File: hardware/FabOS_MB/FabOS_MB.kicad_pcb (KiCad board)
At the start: 4 copper layers, 68 x 68 mm, 117 parts, among them J201 USB_A, J301 RJ45, J401 USB_C_Receptacle, J601 Conn_ST_STDC14, SW601 boot, SW602 SW_Push, SW603 SW_Push, SW604 SW_Push, SW605 SW_Push, U201 NCV7329, U301 LAN8742A, U302 CND-tek B1601S, U303 USBLC6-4SC6, U401 USBLC6-2SC6, U501 TDPOWER TAS12-5-W2, U502 TPS563201, U601 STM32F407VETx, Y301 Crystal_GND24

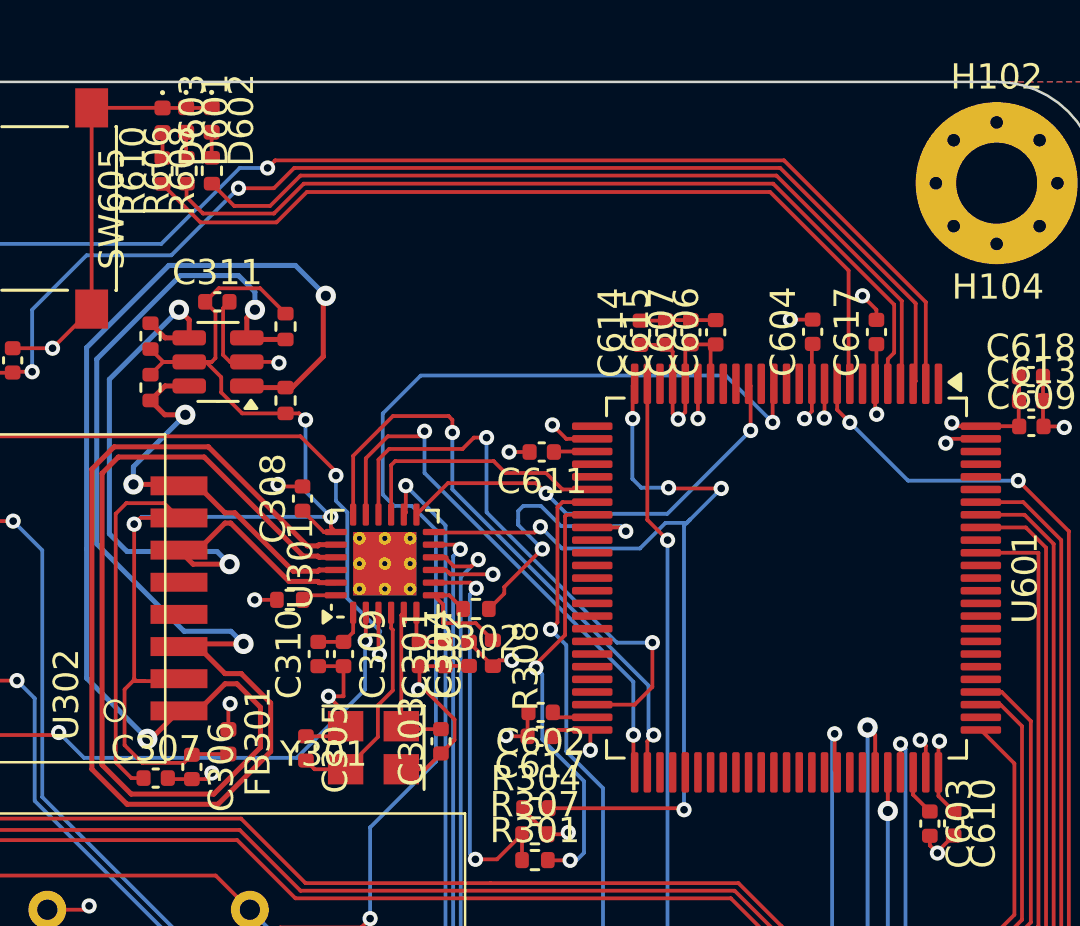
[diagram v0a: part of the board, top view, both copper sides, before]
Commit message: update
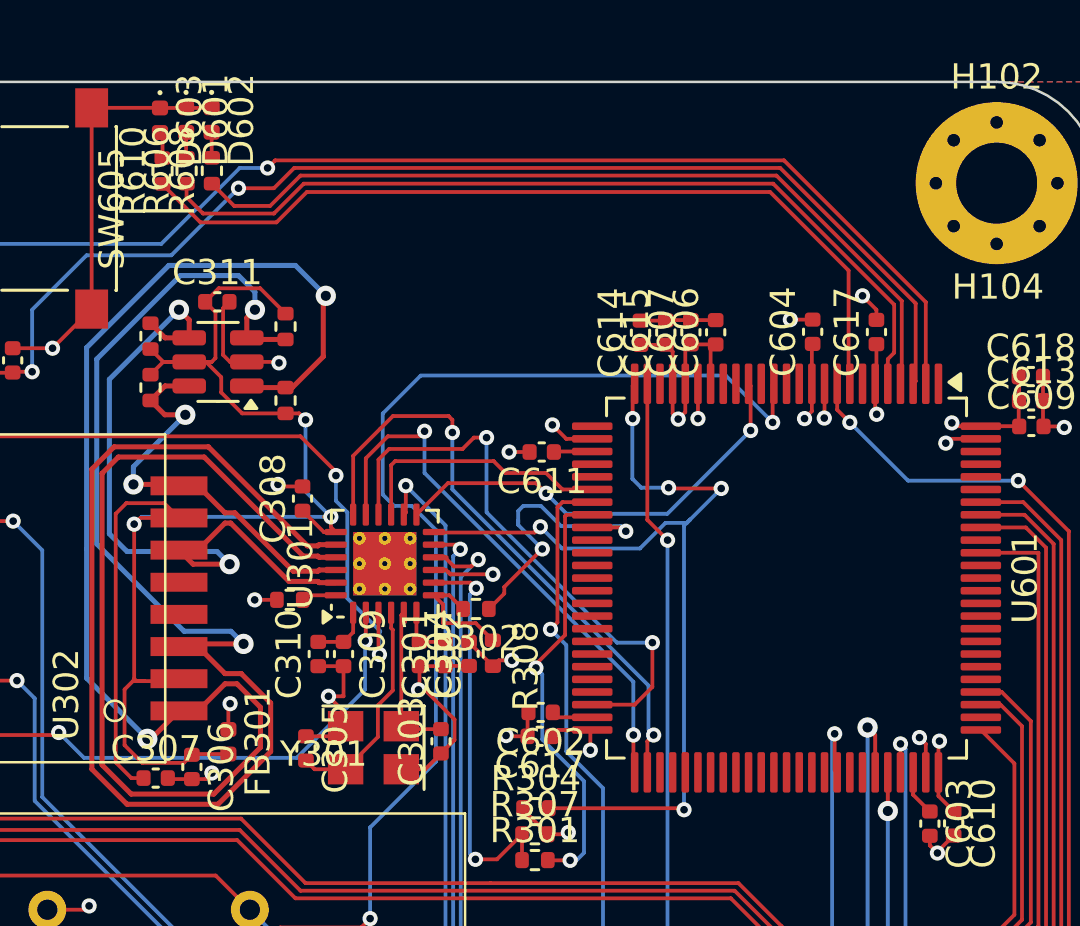
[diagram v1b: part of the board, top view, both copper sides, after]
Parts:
- moved D603 0.10 mm to (127.0, 97.5)
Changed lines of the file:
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@@
 	(footprint "Diode_SMD:D_0402_1005Metric"
 		(layer "F.Cu")
-		(at 127.05 97.515 -90)
+		(at 126.95 97.515 -90)
 		(descr "Diode SMD 0402 (1005 Metric), square (rectangular) end terminal, IPC_7351 nominal, (Body size source: http://www.tortai-tech.com/upload/download/2011102023233369053.pdf), generated with kicad-footprint-generator")
 		(tags "diode")
@@
 	)
 	(segment
+		(start 156.95 121.9)
+		(end 157.2 122.15)
+		(width 0.15)
+		(layer "F.Cu")
+		(net 2)
+	)
+	(segment
 		(start 129.693749 104.6875)
 		(end 129.441749 104.9395)
@@
 	)
 	(segment
-		(start 157.2 123.275)
-		(end 157.2 122.22)
-		(width 0.15)
-		(layer "F.Cu")
-		(net 2)
-	)
-	(segment
 		(start 107.25 154.99)
 		(end 106.34 154.99)
@@
 	)
 	(segment
+		(start 157.2 122.15)
+		(end 157.2 123.275)
+		(width 0.15)
+		(layer "F.Cu")
+		(net 2)
+	)
+	(segment
 		(start 153.2 107.925)
 		(end 153.2 109.27)
@@
 	)
 	(segment
-		(start 157.2 122.22)
-		(end 156.98 122)
-		(width 0.15)
-		(layer "F.Cu")
-		(net 2)
-	)
-	(segment
 		(start 143 149.55)
 		(end 143.2 149.35)
@@
 	)
 	(via
-		(at 156.98 122)
+		(at 156.95 121.9)
 		(size 0.6)
 		(drill 0.3)
@@
 			)
 		)
+	)
+	(zone
+		(net 2)
+		(net_name "GND")
+		(layer "In1.Cu")
+		(hatch edge 0.5)
+		(priority 3)
+		(connect_pads
+			(clearance 0.5)
+		)
+		(min_thickness 0.25)
+		(filled_areas_thickness no)
+		(fill yes
+			(thermal_gap 0.5)
+			(thermal_bridge_width 0.5)
+		)
+		(polygon
+			(pts
+				(xy 96 96) (xy 96 164) (xy 164 164) (xy 164 96)
+			)
+		)
